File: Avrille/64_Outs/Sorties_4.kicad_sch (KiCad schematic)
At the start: 49 parts, among them Q18 TIP127, Q19 TIP127, Q2 TIP127, Q50 TIP127, Q51 TIP127, Q52 TIP127, Q53 TIP127, Q79 TIP127, U44 ULN2803A

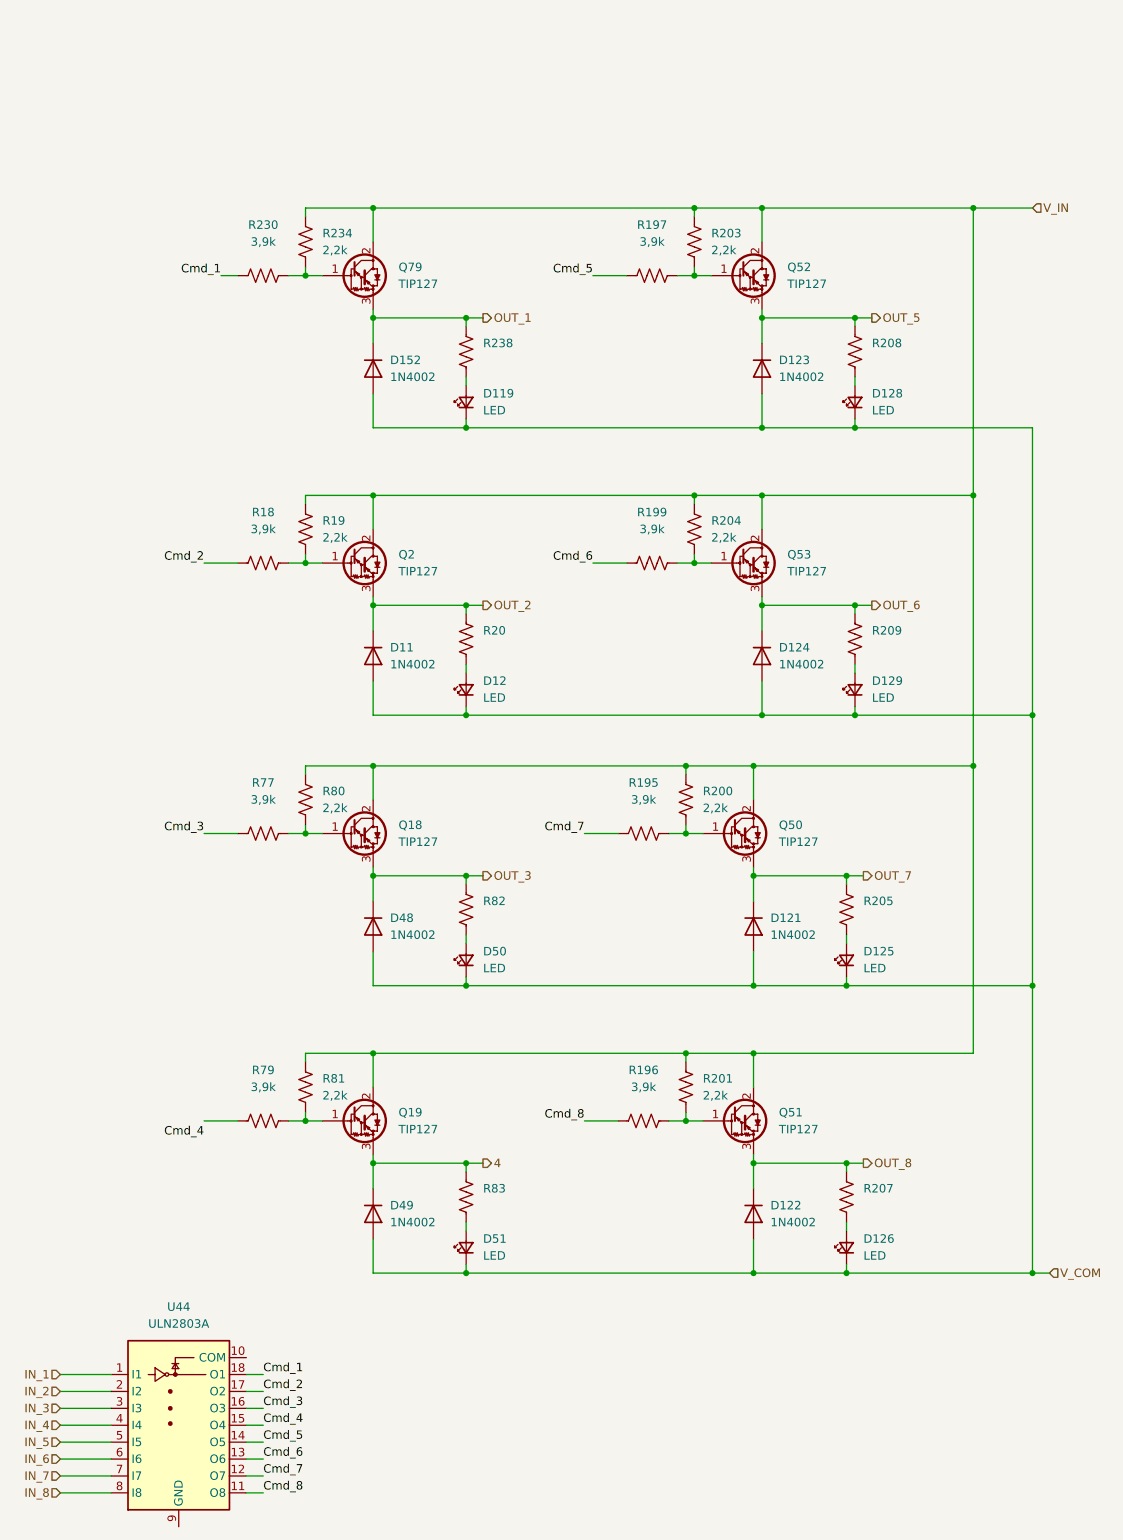
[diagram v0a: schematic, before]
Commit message: reset
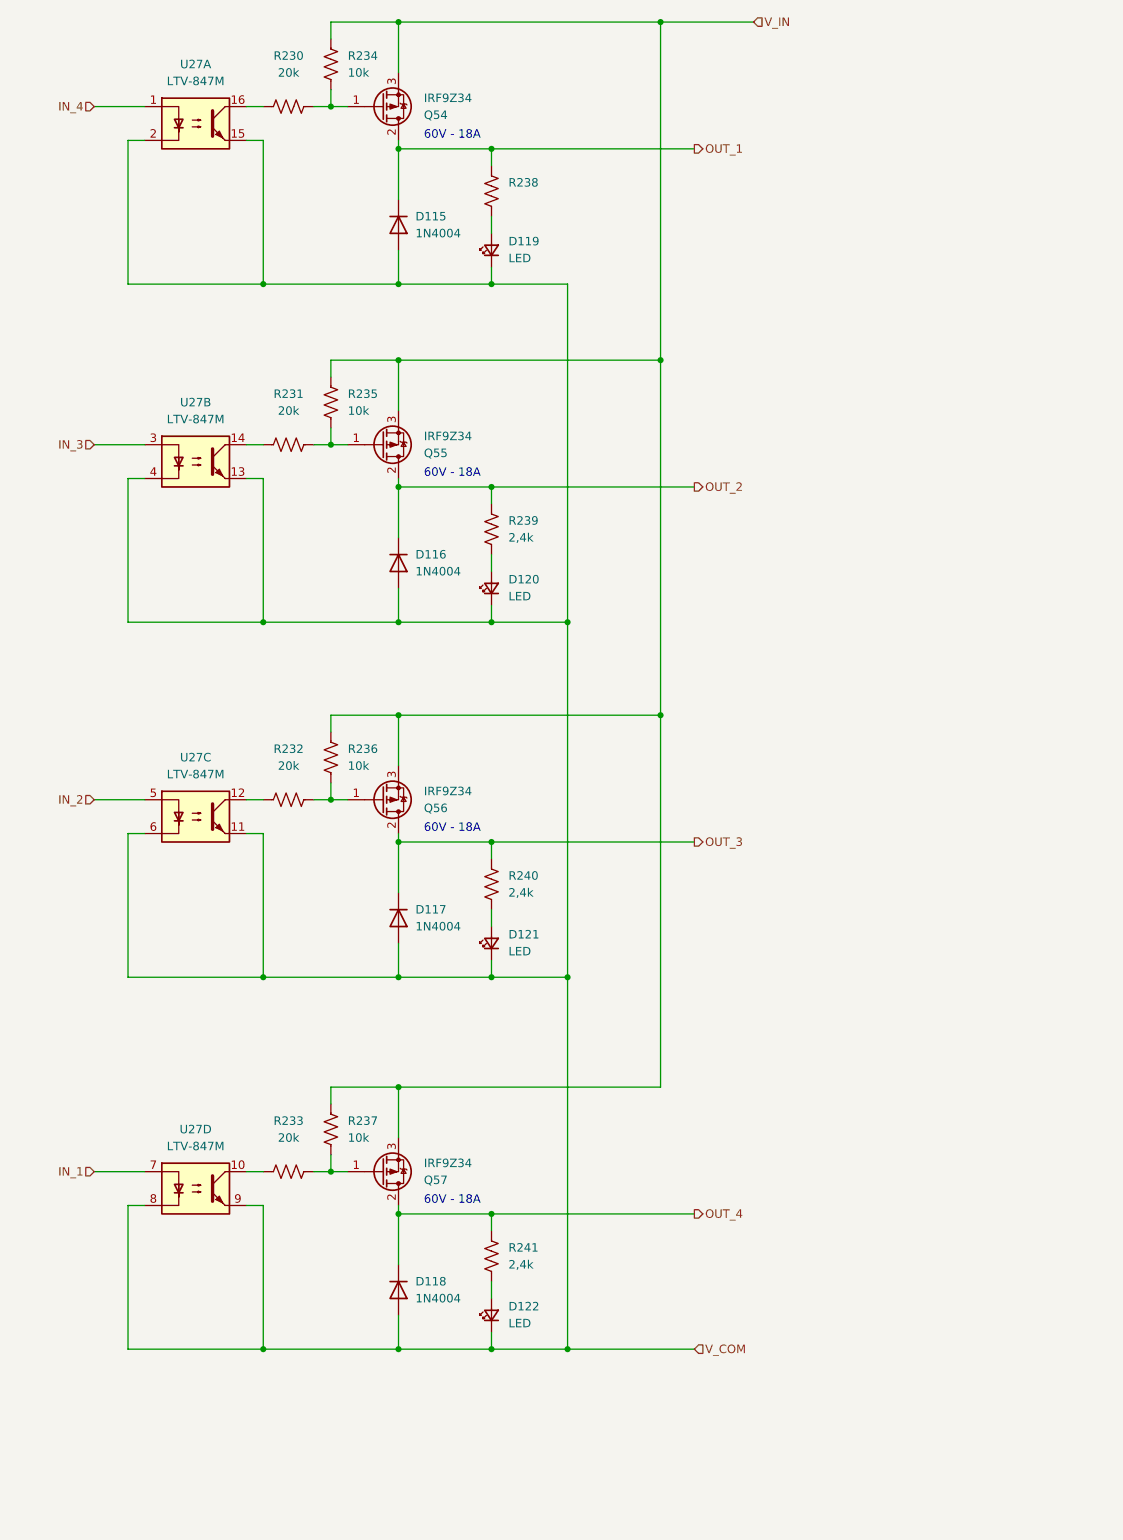
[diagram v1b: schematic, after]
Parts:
- removed D11, D121, D122, D123, D124, D152, D48, D49: 1N4002, Diode_THT:D_DO-41_SOD81_P10.16mm_Horizontal, symbol Diode:1N4002
- removed D12, D125, D126, D128, D129, D50, D51: LED, LED_SMD:LED_PLCC-2_3.4x3.0mm_AK, symbol Device:LED_Small
- removed Q18, Q19, Q2, Q50, Q51, Q52, Q53, Q79: TIP127, Package_TO_SOT_THT:TO-220-3_Vertical, symbol Transistor_BJT:TIP127
- removed R18, R195, R196, R197, R199, R77, R79: 3,9k, Resistor_THT:R_Axial_DIN0207_L6.3mm_D2.5mm_P10.16mm_Horizontal, symbol Device:R_US
- removed R19, R20, R200, R201, R203, R204, R205, R207, R208, R209, R80, R81, R82, R83: 2,2k, Resistor_THT:R_Axial_DIN0207_L6.3mm_D2.5mm_P10.16mm_Horizontal, symbol Device:R_US
- removed U44: ULN2803A, symbol Transistor_Array:ULN2803A
- added D115, D116, D117, D118: 1N4004, Diode_THT:D_DO-41_SOD81_P10.16mm_Horizontal, symbol Diode:1N4004
- added D120, D121, D122: LED, LED_THT:LED_D1.8mm_W3.3mm_H2.4mm, symbol Device:LED_Small
- added Q54, Q55, Q56, Q57: IRF9Z34, Package_TO_SOT_THT:TO-220-3_Vertical, symbol Transistor_FET:IRF4905
- added R231, R232, R233: 20k, Resistor_THT:R_Axial_DIN0207_L6.3mm_D2.5mm_P10.16mm_Horizontal, symbol Device:R_US
- added R235, R236, R237: 10k, Resistor_THT:R_Axial_DIN0207_L6.3mm_D2.5mm_P10.16mm_Horizontal, symbol Device:R_US
- added R239, R240, R241: 2,4k, Resistor_THT:R_Axial_DIN0207_L6.3mm_D2.5mm_P10.16mm_Horizontal, symbol Device:R_US
- added U27: LTV-847M, Package_DIP:DIP-16_W7.62mm, symbol Isolator:LTV-847M
- D119: footprint LED_SMD:LED_PLCC-2_3.4x3.0mm_AK -> LED_THT:LED_D1.8mm_W3.3mm_H2.4mm
- R230: value 3,9k -> 20k
- R234: value 2,2k -> 10k
- R238: value 2,2k -> 2,4k
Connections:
- net IN_1: now also U27.7
- net IN_2: now also U27.5
- net IN_3: now also U27.3
- net IN_4: now also U27.1
- net OUT_1: now also D115.1 (K), Q54.2 (D)
- net OUT_2: now also D116.1 (K), Q55.2 (D), R239.1
- net OUT_3: now also D117.1 (K), Q56.2 (D), R240.1
- net V_COM: now also D115.2 (A), D116.2 (A), D117.2 (A), D118.2 (A), D120.1 (K), D121.1 (K), D122.1 (K), U27.11, U27.13, U27.15, U27.2, U27.4, U27.6, U27.8, U27.9
- net V_IN: now also Q54.3 (S), Q55.3 (S), Q56.3 (S), Q57.3 (S), R235.1, R236.1, R237.1
- net at R230.1, R234.2: now also Q54.1 (G)
- net Cmd_1: no longer names the net of R230.2
- net Cmd_1: now also U27.16
- new net: Q57.1 (G), R233.1, R237.2
- new net: D122.2 (A), R241.2
- new net: R231.2, U27.14
- new net: Q56.1 (G), R232.1, R236.2
- new net: D121.2 (A), R240.2
- new net: R233.2, U27.10
- new net: D120.2 (A), R239.2
- new net: R232.2, U27.12
- new net: Q55.1 (G), R231.1, R235.2
- new net OUT_4: D118.1 (K), Q57.2 (D), R241.1
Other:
- note added: "60V - 18A"
- moved on the sheet: D119, R230, R234, R238
